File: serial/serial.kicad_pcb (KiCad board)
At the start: 2 copper layers, 73.7 x 56.1 mm, 36 parts, among them J1 Conn_02x20_Odd_Even, J2 D-SUB Male 9 pins, J3 Conn_01x06_Male, U1 74LS30, U2 74LS02, U3 74LS02, U4 MC6850, U5 CD4060BE, U6 MAX232, Y1 4.0Mhz

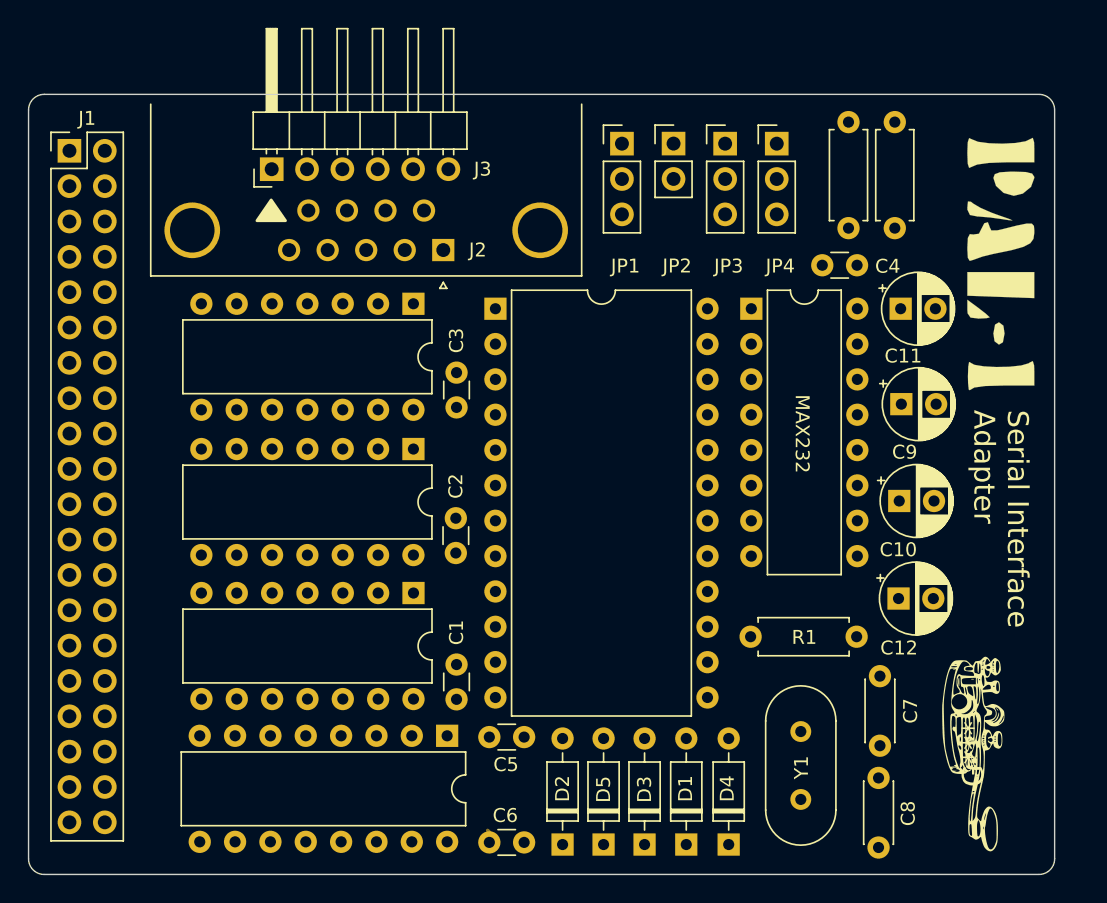
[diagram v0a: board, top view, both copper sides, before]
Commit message: Route pcb
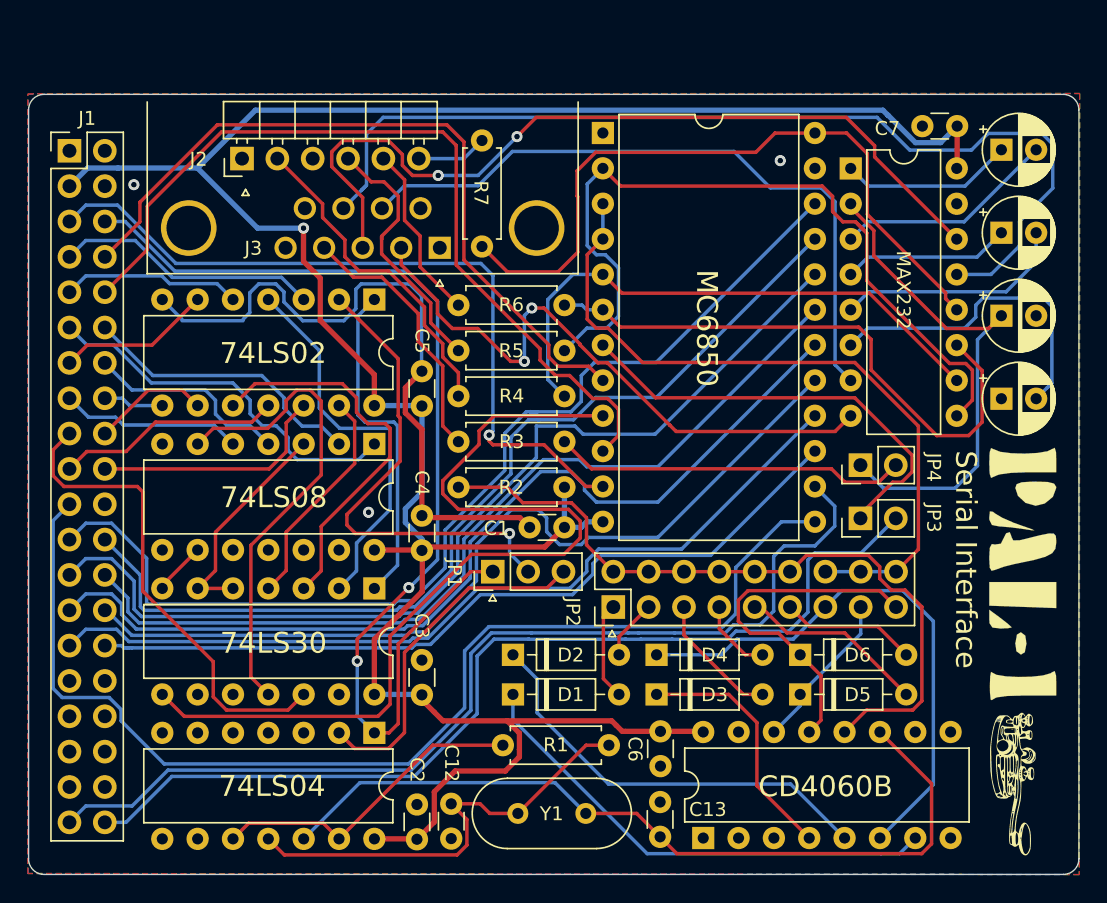
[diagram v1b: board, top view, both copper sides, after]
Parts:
- removed the C7 at (160.9, 112.6)
- removed the C8 at (160.8, 124.9)
- removed the J2 at (129.5, 81.9)
- removed the R1 at (162.0, 80.4)
- removed the R1 at (159.2, 109.7)
- removed the U3 at (127.4, 96.2)
- added C12: 33pF, Capacitor_THT:C_Disc_D3.0mm_W1.6mm_P2.50mm, F.Cu at (130.1, 124.2)
- added C13: 33pF, Capacitor_THT:C_Disc_D3.0mm_W1.6mm_P2.50mm, F.Cu at (145.1, 121.6)
- added C4: 0.1uF, Capacitor_THT:C_Disc_D3.0mm_W1.6mm_P2.50mm, F.Cu at (128.0, 101.0)
- added D6: 1N4148, Diode_THT:D_DO-35_SOD27_P7.62mm_Horizontal, F.Cu at (155.2, 111.0)
- added J3: DB9_Male, Connector_Dsub:DSUB-9_Male_Horizontal_P2.77x2.84mm_EdgePinOffset7.70mm_Housed_MountingHolesOffset9.12mm, F.Cu at (129.2, 81.8)
- added R1: 2K2, Resistor_THT:R_Axial_DIN0207_L6.3mm_D2.5mm_P7.62mm_Horizontal, F.Cu at (141.4, 117.5)
- added R3: 2K7, Resistor_THT:R_Axial_DIN0207_L6.3mm_D2.5mm_P7.62mm_Horizontal, F.Cu at (130.6, 95.7)
- added R4: 2K2, Resistor_THT:R_Axial_DIN0207_L6.3mm_D2.5mm_P7.62mm_Horizontal, F.Cu at (130.6, 92.4)
- added R5: 2K2, Resistor_THT:R_Axial_DIN0207_L6.3mm_D2.5mm_P7.62mm_Horizontal, F.Cu at (130.6, 89.2)
- added R6: 2K2, Resistor_THT:R_Axial_DIN0207_L6.3mm_D2.5mm_P7.62mm_Horizontal, F.Cu at (130.6, 85.9)
- added R7: 2K2, Resistor_THT:R_Axial_DIN0207_L6.3mm_D2.5mm_P7.62mm_Horizontal, F.Cu at (132.3, 74.1)
- added U4: 74LS08, Package_DIP:DIP-14_W7.62mm, F.Cu at (124.5, 95.9)
- added U6: 74LS04, Package_DIP:DIP-14_W7.62mm, F.Cu at (124.5, 116.6)
- JP2: value Jumper_2_Open -> Conn_02x09_Odd_Even; footprint Connector_PinHeader_2.54mm:PinHeader_1x02_P2.54mm_Vertical -> Connector_PinHeader_2.54mm:PinHeader_2x09_P2.54mm_Vertical
- JP3, JP4: value Jumper_3_Bridged12 -> Jumper_2_Open; footprint Connector_PinHeader_2.54mm:PinHeader_1x03_P2.54mm_Vertical -> Connector_PinHeader_2.54mm:PinHeader_1x02_P2.54mm_Vertical
- moved C7 58.9 mm to (163.9, 73.0), turned to 0 degrees
- moved R2 33.7 mm to (130.6, 99.0), turned to 0 degrees
- moved JP2 33.6 mm to (141.7, 107.6), turned to 90 degrees
- moved JP1 32.1 mm to (133.1, 105.1), turned to 90 degrees
- moved C6 29.7 mm to (145.1, 119.0)
- moved JP3 28.6 mm to (159.5, 101.2), turned to 90 degrees
- moved C1 28.2 mm to (135.7, 101.9)
- moved JP4 23.9 mm to (159.5, 97.4), turned to 90 degrees
- moved G*** 22.3 mm to (171.1, 105.1)
- moved C9 20.6 mm to (169.6, 80.7)
- moved Y1 20.4 mm to (134.9, 122.4), turned to 0 degrees
- moved U2 19.8 mm to (148.2, 124.2), turned to 90 degrees
- moved C8 19.6 mm to (169.6, 74.7)
- moved D5 17.8 mm to (155.2, 113.9), turned to 0 degrees
- moved D1 16.5 mm to (134.5, 113.9), turned to 0 degrees
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- renumbered C4 to C1, C11 to C10, C12 to C11, C5 to C2, C1 to C3, C2 to C5, C3 to C6, C6 to C7, C9 to C8, C10 to C9, J3 to J2, U4 to U1, U5 to U2, U1 to U3, U2 to U5, U6 to U7
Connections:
- C10 pad 1: Net-(C11-Pad1) -> Net-(C10-Pad1)
- D3 pad 2: Net-(D1-Pad2) -> Net-(D3-Pad2)
- D5 pad 2: Net-(D2-Pad2) -> Net-(D5-Pad2)
- J2 pad 2: /RTS# -> Net-(J2-Pad2)
- J2 pad 4: /Rx_D -> Net-(J2-Pad4)
- J2 pad 5: /Tx_D -> Net-(J2-Pad5)
- J2 pad 6: /CTS# -> Net-(J2-Pad6)
- JP1 pad 1: Net-(JP1-Pad1) -> A1
- JP1 pad 3: A1 -> Net-(JP1-Pad3)
- JP2 pad 1: Net-(JP2-Pad1) -> Net-(D1-Pad2)
- JP2 pad 2: IRQ -> Net-(JP2-Pad10)
- JP3 pad 1: Net-(D4-Pad1) -> Net-(JP3-Pad1)
- JP3 pad 2: CLK -> IRQ
- JP4 pad 1: Net-(D1-Pad2) -> Net-(C10-Pad1)
- JP4 pad 2: Net-(D4-Pad2) -> Net-(JP4-Pad2)
- R2 pad 1: Net-(D4-Pad2) -> Net-(JP2-Pad10)
- U1 pad 10: A3 -> A5
- U1 pad 14: PHI2 -> PHI1
- U1 pad 7: Net-(JP2-Pad1) -> Net-(JP3-Pad1)
- U1 pad 8: A5 -> A3
- U2 pad 10: Net-(C7-Pad2) -> unconnected-(U2-Pad10)
- U2 pad 11: Net-(C8-Pad2) (its old number) -> Net-(C13-Pad2)
- U2 pad 12: Net-(D4-Pad2) -> Net-(JP2-Pad10)
- U2 pad 13: unconnected-(U5-Pad13) -> Net-(D6-Pad1)
- U3 pad 1: Net-(JP1-Pad2) -> Net-(U3-Pad1)
- U3 pad 2: Net-(U1-Pad2) -> Net-(U3-Pad2)
- U3 pad 3: Net-(U1-Pad3) -> Net-(U3-Pad3)
- U3 pad 4: Net-(U1-Pad4) -> Net-(U3-Pad4)
- U3 pad 5: Net-(U1-Pad5) -> Net-(U3-Pad5)
- U3 pad 6: Net-(U1-Pad6) -> Net-(U3-Pad5)
- U5 pad 1: Net-(U1-Pad2) -> Net-(U3-Pad1)
- U5 pad 10: Net-(U1-Pad4) -> Net-(U3-Pad3)
- U5 pad 13: Net-(U1-Pad5) -> Net-(U3-Pad4)
- U5 pad 2: GND -> Net-(JP1-Pad2)
- U5 pad 4: Net-(U1-Pad3) -> Net-(U3-Pad2)
- U7 pad 10: /Tx_D -> /RTS#
- U7 pad 11: /RTS# -> /Tx_D
- U7 pad 12: /Rx_D -> /CTS#
- U7 pad 13: RXD -> /CTS
- U7 pad 14: RTS -> /TXD
- U7 pad 2: Net-(C11-Pad1) -> Net-(C10-Pad1)
- U7 pad 7: TXD -> /RTS
- U7 pad 8: CTS -> /RXD
- U7 pad 9: /CTS# -> /Rx_D
- Y1 pad 1: Net-(C8-Pad2) (its old number) -> Net-(C12-Pad2)
- Y1 pad 2: Net-(C7-Pad2) -> Net-(C13-Pad2)
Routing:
- net VCC: track 1.03 -> 182.7 mm, vias 0 -> 1
- net R/~{W}: track 0.00 -> 82.8 mm
- net A1: track 0.00 -> 76.9 mm, vias 0 -> 2
- net D0: track 0.00 -> 75.1 mm
- net PHI1: track 0.00 -> 72.0 mm
- net /CTS: track 0.00 -> 71.7 mm
- net IRQ: track 0.00 -> 70.5 mm
- net D2: track 0.00 -> 70.5 mm
- net D1: track 0.00 -> 68.7 mm
- net D4: track 0.00 -> 67.5 mm
- net Net-(U1-Pad9): track 0.00 -> 65.7 mm
- net D3: track 0.00 -> 64.3 mm
- net D5: track 0.00 -> 63.5 mm
- net D6: track 0.00 -> 61.6 mm
- net A5: track 0.00 -> 60.8 mm
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- added copper zone on B.Cu, net GND
- added copper zone on F.Cu, net GND
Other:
- board size 73.7 x 56.1 mm -> 75.5 x 56.1 mm
- board text added: "74LS02"
- board text added: "74LS04"
- board text added: "74LS08"
- board text added: "74LS30"
- board text added: "CD4060B"
- board text added: "MC6850"
- board text added: "Serial Interface"
- board text removed: "Serial Interface Adapter"
